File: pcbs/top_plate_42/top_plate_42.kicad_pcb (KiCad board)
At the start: 2 copper layers, 131.8 x 95.3 mm, 6 parts

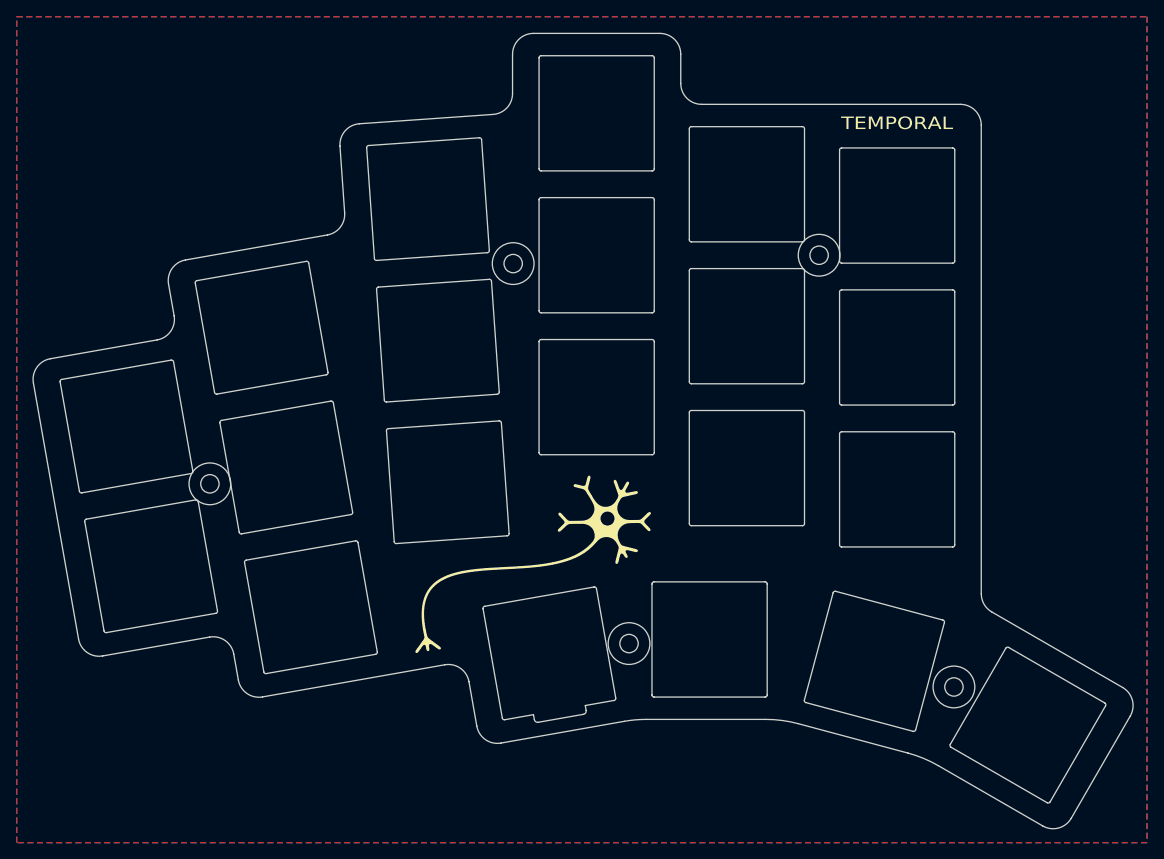
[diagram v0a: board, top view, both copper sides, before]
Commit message: update generated files
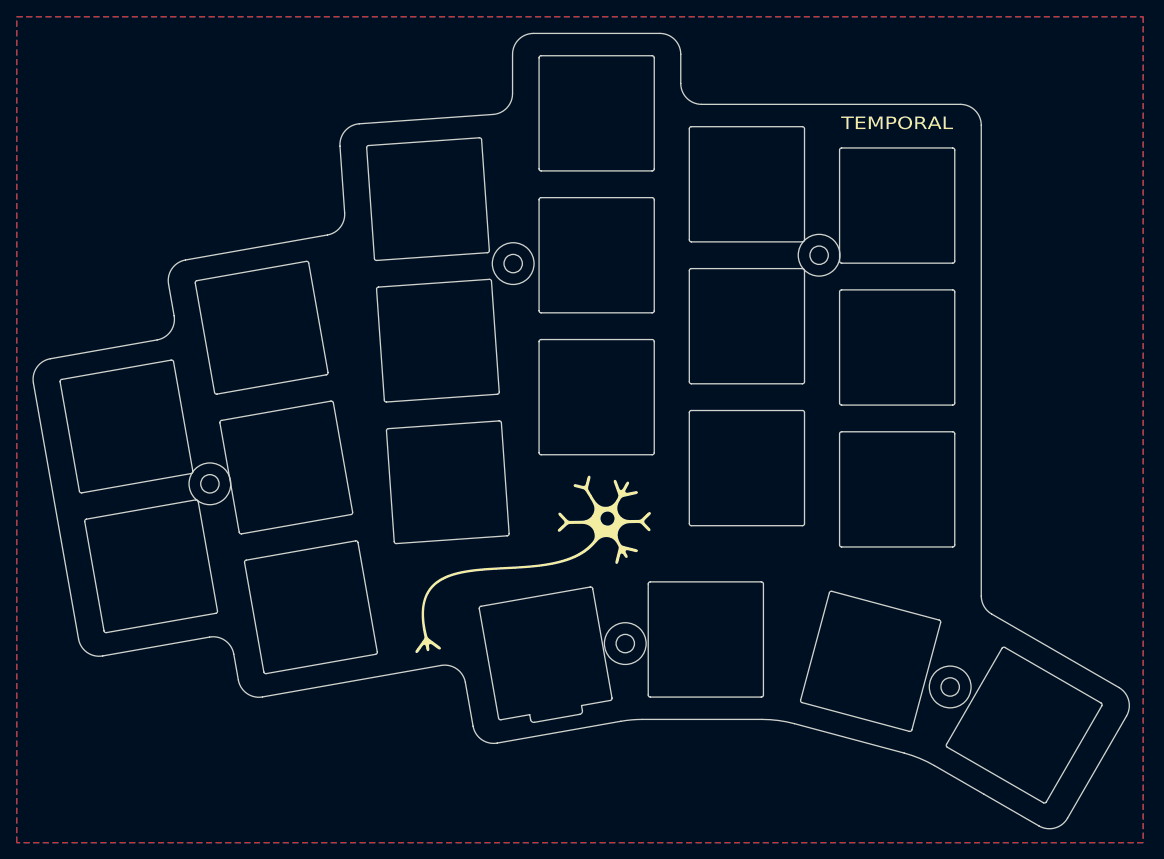
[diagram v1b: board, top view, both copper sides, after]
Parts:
- moved MH3 0.45 mm to (142.8, 97.7)
- moved MH4 0.45 mm to (103.9, 92.5)
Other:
- board size 131.8 x 95.3 mm -> 131.3 x 95.3 mm
